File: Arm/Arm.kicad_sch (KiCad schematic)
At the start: 57 parts, among them J10 SparkMAX XT60 F, J11 CAN OUT, J12 SparkMAX XT60 F, J13 SparkMAX XT60 F, J14 Encoder 0, J2 Encoder Bundle, J3 CAN IN, J4 5V Swtich Power, J5 Power IN XT60 M, J6 SparkMAX XT60 F, J7 Power OUT XT60 F, J8 Digit 12V, J9 CANBUS, M1 Fan, M2 Fan, U4 TJA1051T, U5 ESP32-S3-DevKitC, U9 MCP251863T-E-9PX, Y3 40Mhz Crystal

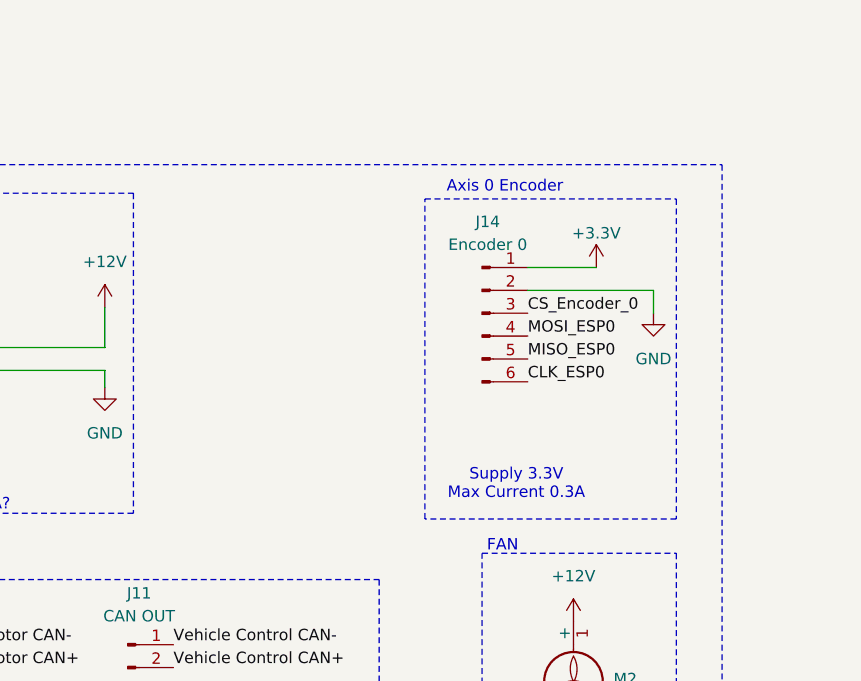
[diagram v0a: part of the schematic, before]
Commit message: 2/3 Final Changes
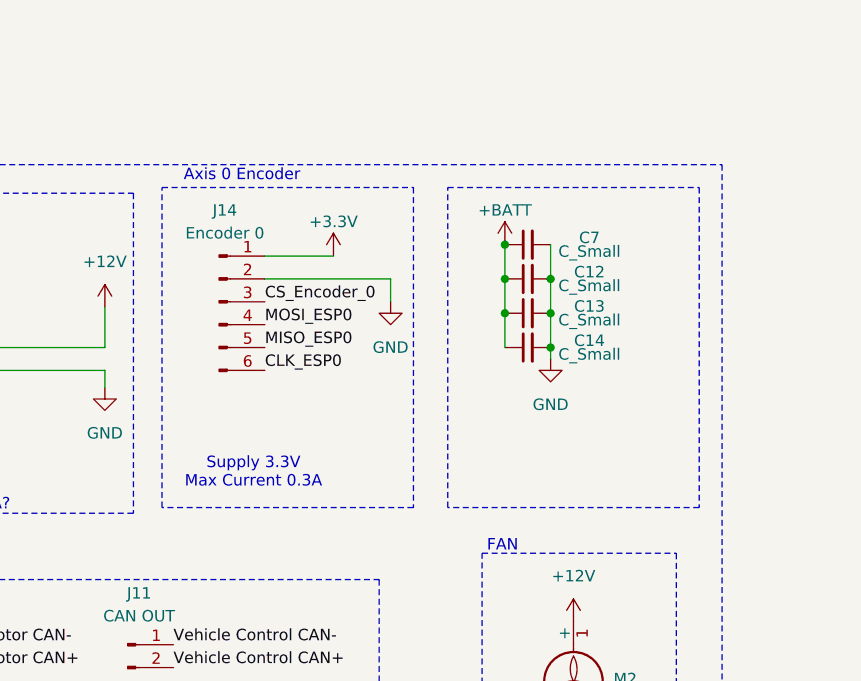
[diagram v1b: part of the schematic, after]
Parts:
- added C12, C13, C14, C7: C_Small, Capacitor_SMD:C_Elec_4x5.8, symbol Device:C_Small
- J10, J13: footprint Connector_AMASS:AMASS_XT60PW-F_1x02_P7.20mm_Horizontal -> Connector_AMASS:AMASS_XT60-F_1x02_P7.20mm_Vertical
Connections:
- net +BATT: now also C12.1, C13.1, C14.1, C7.1
- net GND: now also C12.2, C13.2, C14.2, C7.2
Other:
- moved on the sheet: J14

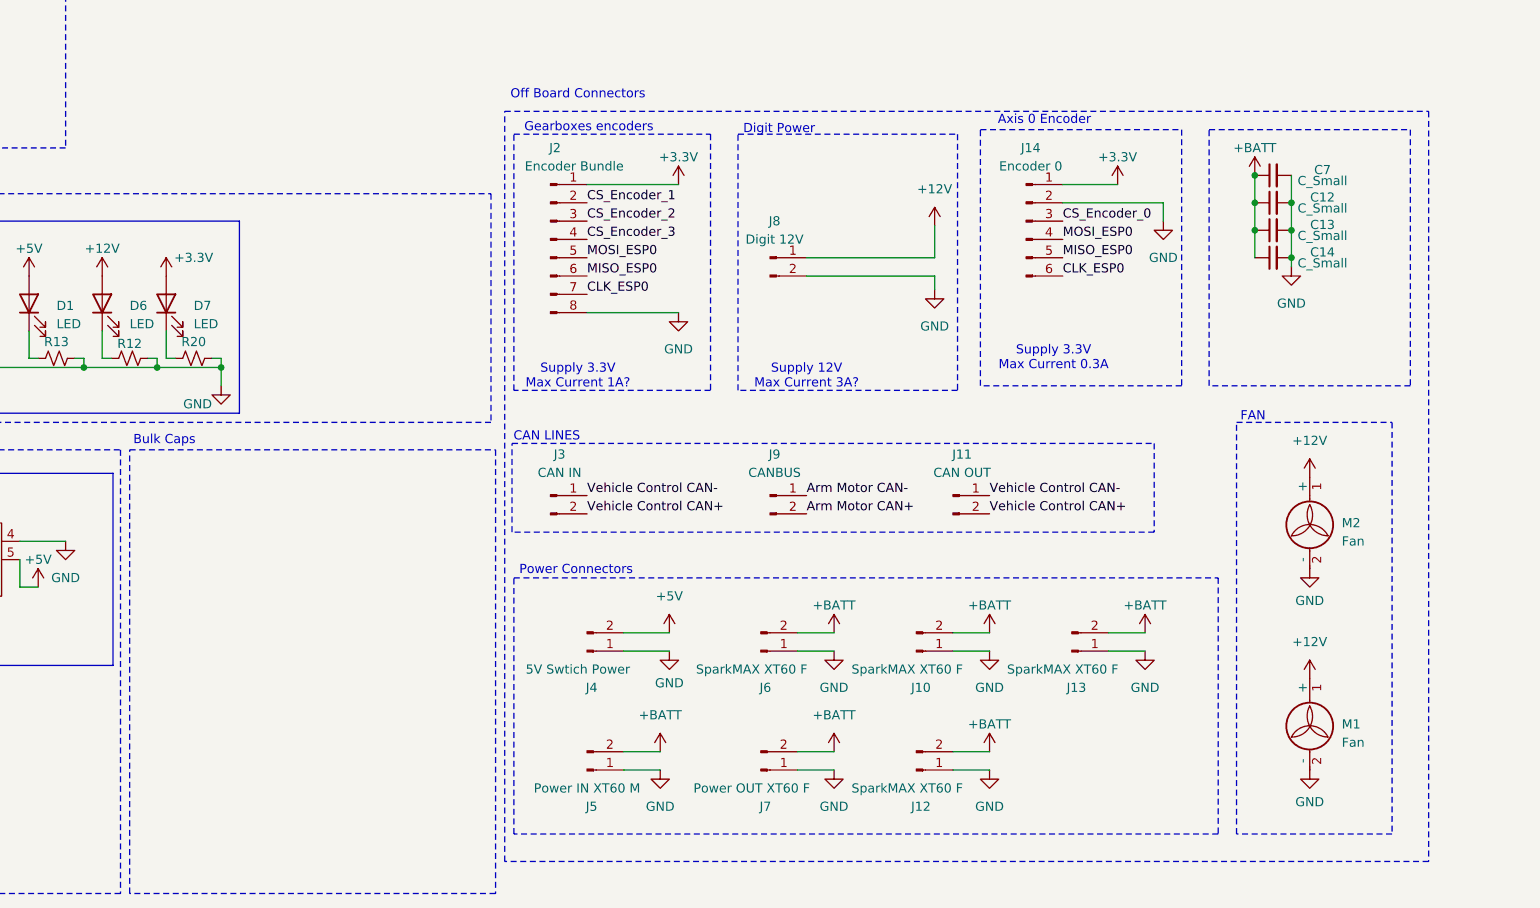
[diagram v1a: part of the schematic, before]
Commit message: Final Part 3
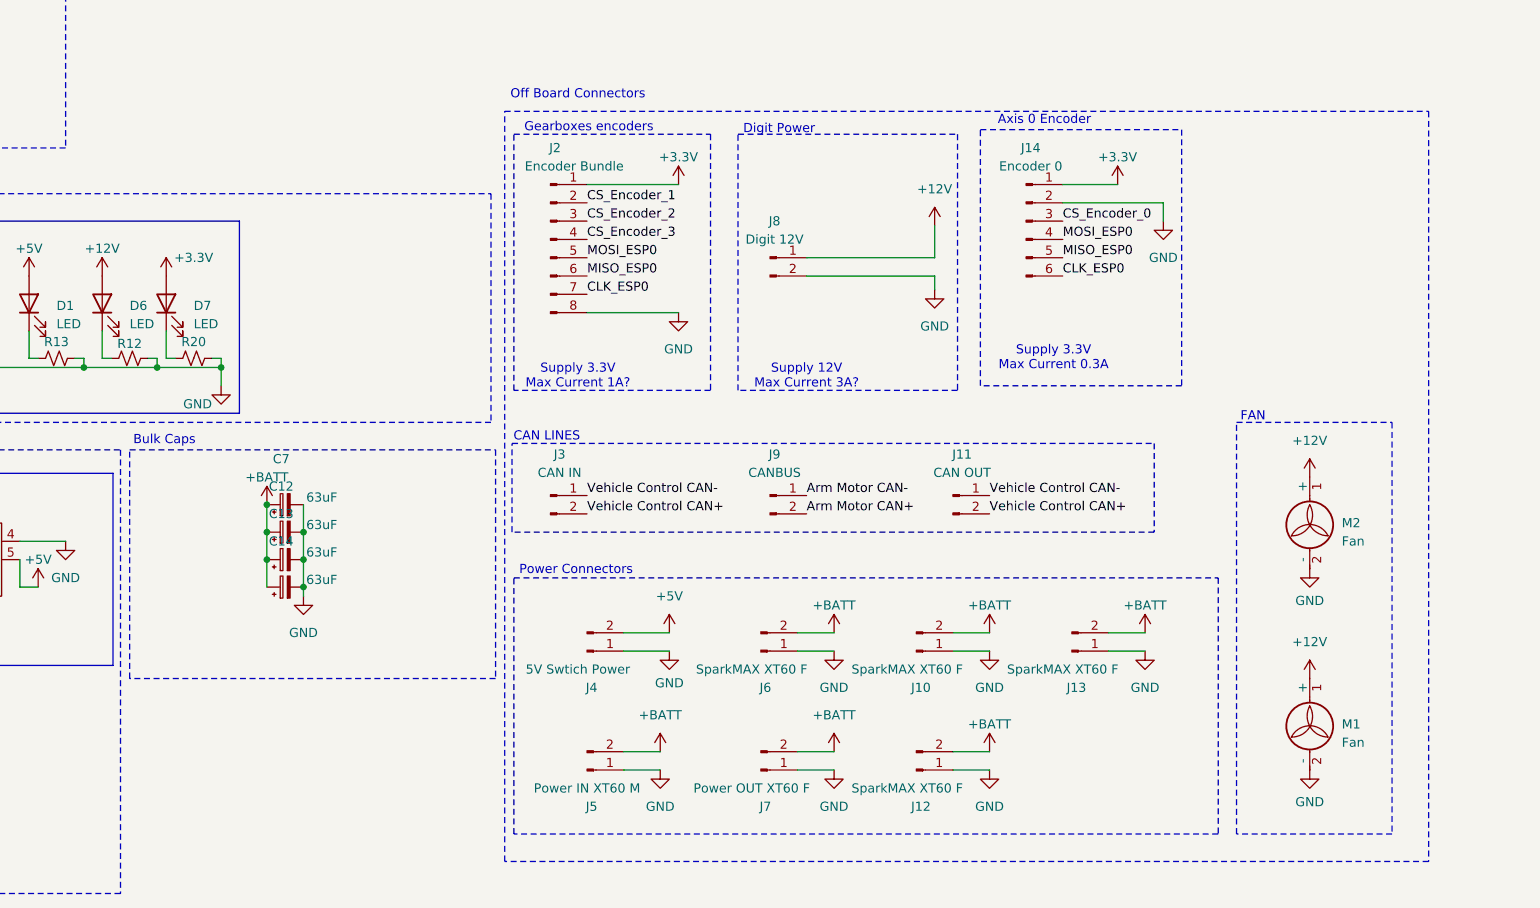
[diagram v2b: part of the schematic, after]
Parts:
- removed C12, C13, C14, C7: C_Small, Capacitor_SMD:C_Elec_4x5.8, symbol Device:C_Small
- added C12, C13, C14, C7: 63uF, Capacitor_SMD:CP_Elec_6.3x7.7, symbol Device:C_Polarized_Small
- J12, J6: footprint Connector_AMASS:AMASS_XT60PW-F_1x02_P7.20mm_Horizontal -> Connector_AMASS:AMASS_XT60-F_1x02_P7.20mm_Vertical
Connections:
- net +BATT: now also C12.1, C13.1, C14.1, C7.1
- net GND: now also C12.2, C13.2, C14.2, C7.2
